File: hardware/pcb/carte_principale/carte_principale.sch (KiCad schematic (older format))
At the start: 20 parts, among them J1 Arduino_UNO_R3, J2 Conn_01x02, J3 Conn_01x02, P1 TE-FFC-10-0.5, P2 TE-FFC-10-0.5, U1 ESP-WROOM-02, U2 LSM6DS3, U3 BMP280, U5 74AHC1G125, U6 74LS166, U7 LIS2MDL

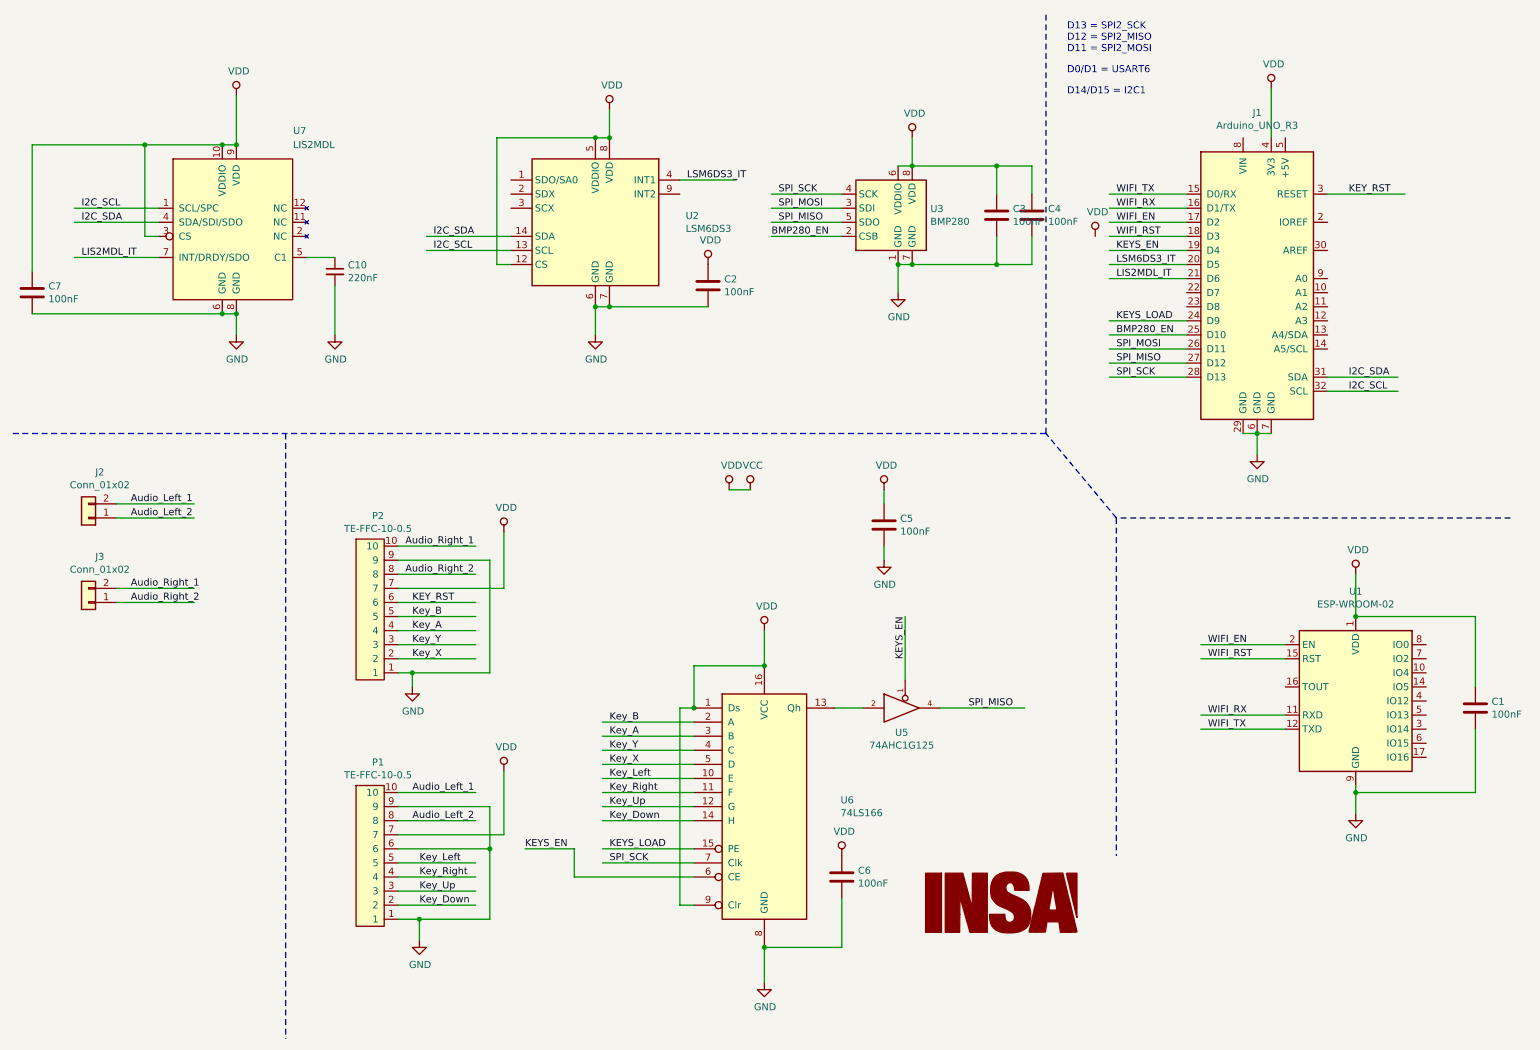
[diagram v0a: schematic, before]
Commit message: sauvegarde intermediaire
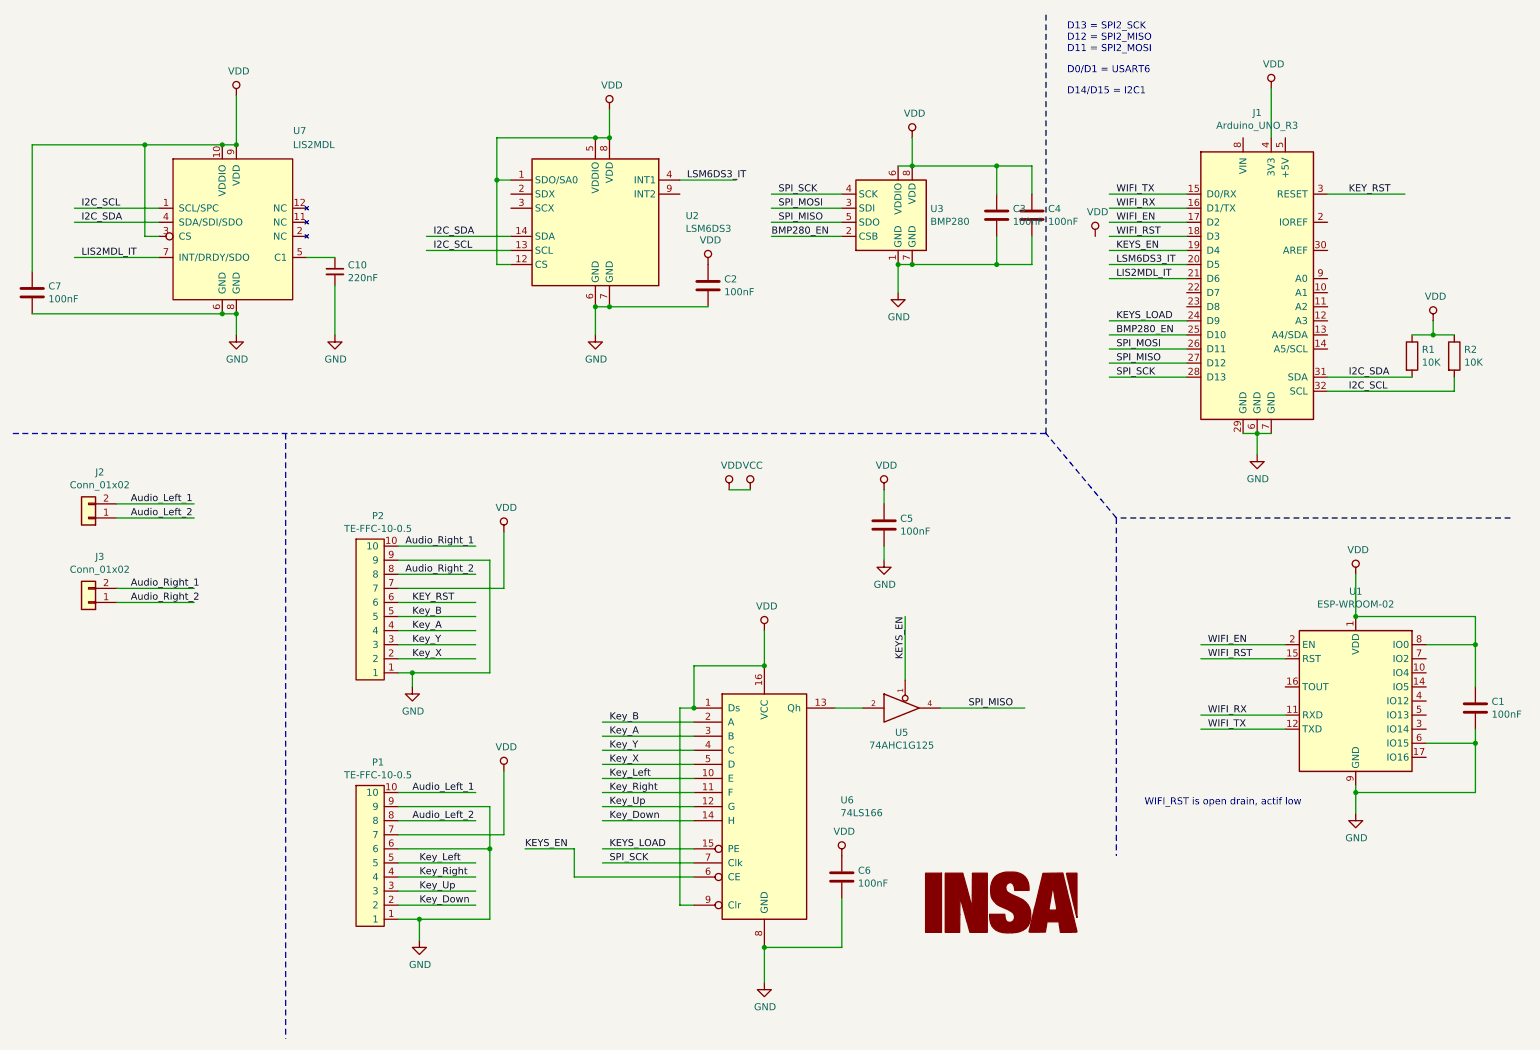
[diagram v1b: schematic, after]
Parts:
- added R1, R2: 10K, Resistor_SMD:R_1206_3216Metric, symbol Device:R
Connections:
- wire segments 133 -> 143
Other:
- note added: "WIFI_RST is open drain, actif low"
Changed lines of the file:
@@
 Title "Carte Principale"
 Date "2019-04-26"
-Rev "02A"
+Rev "02B"
 Comp ""
 Comment1 ""
@@
 D14/D15 = I2C1
 Wire Wire Line
-	9900 3100 10400 3100
-Wire Wire Line
-	9900 3200 10400 3200
-Wire Wire Line
 	8900 1800 8350 1800
 Wire Wire Line
@@
 	4000 1400 4700 1400
 Wire Wire Line
-	4000 1400 4000 2300
+	4000 1400 4000 1700
 Connection ~ 4700 1400
 Wire Wire Line
@@
 	10100 6050 10950 6050
 Wire Wire Line
-	10950 6050 10950 5600
+	10950 6050 10950 5700
 Connection ~ 10100 6050
 Wire Wire Line
 	10100 6050 10100 6000
 Wire Wire Line
-	10950 5300 10950 4800
+	10950 5300 10950 5000
 Wire Wire Line
 	10950 4800 10100 4800
@@
 KEYS_LOAD
 $Comp
-L power:VDD #PWR?
+L power:VDD #PWR0124
 U 1 1 5CE25200
 P 6950 1400
-F 0 "#PWR?" H 6950 1250 50  0001 C CNN
+F 0 "#PWR0124" H 6950 1250 50  0001 C CNN
 F 1 "VDD" H 6967 1573 50  0000 C CNN
 F 2 "" H 6950 1400 50  0001 C CNN
@@
 	1    0    0    -1
 $EndComp
+Wire Wire Line
+	4100 1700 4000 1700
+Connection ~ 4000 1700
+Wire Wire Line
+	4000 1700 4000 2300
+$Comp
+L Device:R R1
+U 1 1 5CE68C07
+P 10500 2950
+F 0 "R1" H 10570 2996 50  0000 L CNN
+F 1 "10K" H 10570 2905 50  0000 L CNN
+F 2 "Resistor_SMD:R_1206_3216Metric" V 10430 2950 50  0001 C CNN
+F 3 "~" H 10500 2950 50  0001 C CNN
+	1    10500 2950
+	1    0    0    -1
+$EndComp
+$Comp
+L Device:R R2
+U 1 1 5CE68CA1
+P 10800 2950
+F 0 "R2" H 10870 2996 50  0000 L CNN
+F 1 "10K" H 10870 2905 50  0000 L CNN
+F 2 "Resistor_SMD:R_1206_3216Metric" V 10730 2950 50  0001 C CNN
+F 3 "~" H 10800 2950 50  0001 C CNN
+	1    10800 2950
+	1    0    0    -1
+$EndComp
+Wire Wire Line
+	10500 2800 10650 2800
+Wire Wire Line
+	10650 2800 10650 2700
+Connection ~ 10650 2800
+Wire Wire Line
+	10650 2800 10800 2800
+Wire Wire Line
+	9900 3100 10500 3100
+Wire Wire Line
+	10800 3200 10800 3100
+Wire Wire Line
+	9900 3200 10800 3200
+$Comp
+L power:VDD #PWR0125
+U 1 1 5CE85BB2
+P 10650 2700
+F 0 "#PWR0125" H 10650 2550 50  0001 C CNN
+F 1 "VDD" H 10667 2873 50  0000 C CNN
+F 2 "" H 10650 2700 50  0001 C CNN
+F 3 "" H 10650 2700 50  0001 C CNN
+	1    10650 2700
+	1    0    0    -1
+$EndComp
+Wire Wire Line
+	10600 5000 10950 5000
+Connection ~ 10950 5000
+Wire Wire Line
+	10950 5000 10950 4800
+Wire Wire Line
+	10600 5700 10950 5700
+Connection ~ 10950 5700
+Wire Wire Line
+	10950 5700 10950 5600
+Text Notes 8600 6150 0    50   ~ 0
+WIFI_RST is open drain, actif low
 $EndSCHEMATC
